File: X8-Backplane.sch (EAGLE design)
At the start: 16 parts, among them IC1 MAX3467CPA, U1 BD6221FSOP, U2 MIC29501-5.0WU, U3 MIC29501-5.0WU

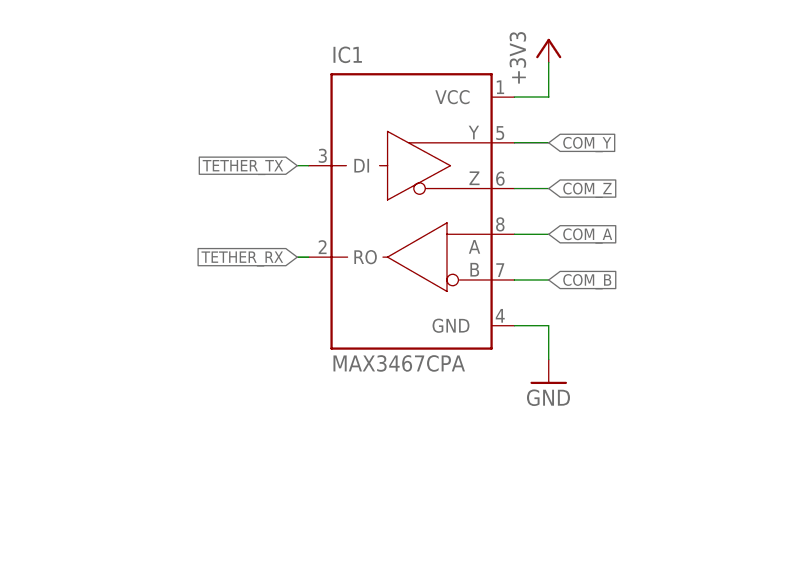
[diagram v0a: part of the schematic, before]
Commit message: finished adding components, added descriptions of pins
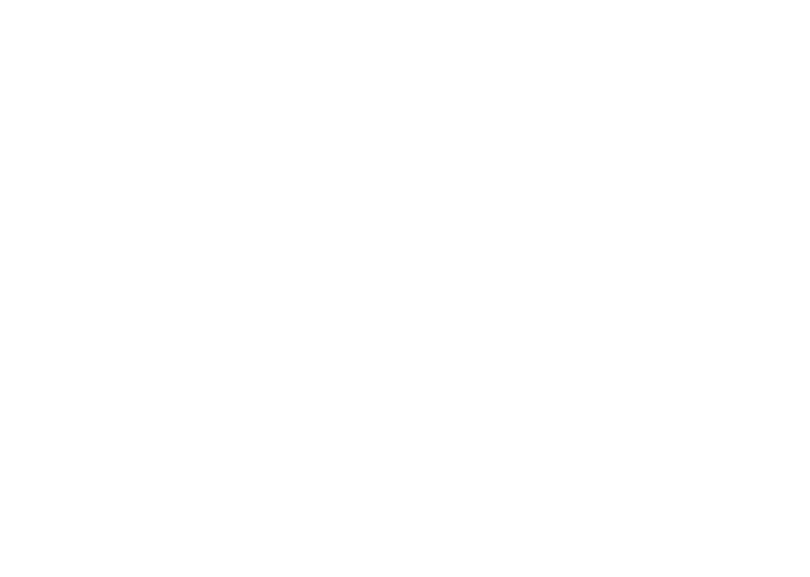
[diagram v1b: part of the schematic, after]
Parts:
- removed IC1: MAX3467CPA, maxim:MAX3467CPA
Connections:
- removed net +3V3: IC1.VCC
- removed net COM_A: IC1.A
- removed net COM_B: IC1.B
- removed net COM_Y: IC1.Y
- removed net COM_Z: IC1.Z
- removed net TETHER_RX: IC1.RO
- removed net TETHER_TX: IC1.DI
- net GND: no longer IC1.GND
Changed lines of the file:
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@@
 <part name="U$3" library="Other" deviceset="BNO055_9DOF_BREAKOUT" device=""/>
 <part name="U$4" library="backplane_to_shield_connector" deviceset="SHIELDCONNECTOR" device=""/>
-<part name="IC1" library="maxim" deviceset="MAX3467*" device="PA" technology="C"/>
-<part name="+3V1" library="supply1" deviceset="+3V3" device=""/>
-<part name="GND1" library="supply1" deviceset="GND" device=""/>
 <part name="U$7" library="test_lib" deviceset="PCA9615" device=""/>
 <part name="U2" library="LDO" deviceset="MIC29501-5.0WU" device=""/>
@@
 <instance part="U$4" gate="G$1" x="373.38" y="91.44"/>
 <instance part="U$4" gate="G$2" x="419.1" y="88.9"/>
-<instance part="IC1" gate="G$1" x="496.57" y="172.72"/>
-<instance part="+3V1" gate="G$1" x="513.08" y="191.77"/>
-<instance part="GND1" gate="1" x="513.08" y="153.67"/>
 <instance part="U$7" gate="G$1" x="408.94" y="165.1"/>
 <instance part="U2" gate="A" x="160.02" y="-40.64"/>
@@
 <nets>
 <net name="GND" class="0">
-<segment>
-<pinref part="IC1" gate="G$1" pin="GND"/>
-<wire x1="509.27" y1="160.02" x2="513.08" y2="160.02" width="0.1524" layer="91"/>
-<wire x1="513.08" y1="160.02" x2="513.08" y2="156.21" width="0.1524" layer="91"/>
-<pinref part="GND1" gate="1" pin="GND"/>
-</segment>
 <segment>
 <pinref part="U2" gate="A" pin="GND"/>
@@
 </segment>
 </net>
-<net name="+3V3" class="0">
-<segment>
-<pinref part="IC1" gate="G$1" pin="VCC"/>
-<wire x1="509.27" y1="185.42" x2="513.08" y2="185.42" width="0.1524" layer="91"/>
-<wire x1="513.08" y1="185.42" x2="513.08" y2="189.23" width="0.1524" layer="91"/>
-<pinref part="+3V1" gate="G$1" pin="+3V3"/>
-</segment>
-</net>
-<net name="TETHER_RX" class="0">
-<segment>
-<pinref part="IC1" gate="G$1" pin="RO"/>
-<wire x1="486.41" y1="167.64" x2="485.14" y2="167.64" width="0.1524" layer="91"/>
-<label x="485.14" y="167.64" size="1.27" layer="95" rot="R180" xref="yes"/>
-</segment>
-</net>
-<net name="TETHER_TX" class="0">
-<segment>
-<label x="485.14" y="177.8" size="1.27" layer="95" rot="R180" xref="yes"/>
-<pinref part="IC1" gate="G$1" pin="DI"/>
-<wire x1="485.14" y1="177.8" x2="486.41" y2="177.8" width="0.1524" layer="91"/>
-</segment>
-</net>
-<net name="COM_A" class="0">
-<segment>
-<pinref part="IC1" gate="G$1" pin="A"/>
-<wire x1="509.27" y1="170.18" x2="513.08" y2="170.18" width="0.1524" layer="91"/>
-<label x="513.08" y="170.18" size="1.27" layer="95" xref="yes"/>
-</segment>
-</net>
-<net name="COM_B" class="0">
-<segment>
-<pinref part="IC1" gate="G$1" pin="B"/>
-<wire x1="509.27" y1="165.1" x2="513.08" y2="165.1" width="0.1524" layer="91"/>
-<label x="513.08" y="165.1" size="1.27" layer="95" xref="yes"/>
-</segment>
-</net>
-<net name="COM_Y" class="0">
-<segment>
-<pinref part="IC1" gate="G$1" pin="Y"/>
-<wire x1="509.27" y1="180.34" x2="513.08" y2="180.34" width="0.1524" layer="91"/>
-<label x="513.08" y="180.34" size="1.27" layer="95" xref="yes"/>
-</segment>
-</net>
-<net name="COM_Z" class="0">
-<segment>
-<pinref part="IC1" gate="G$1" pin="Z"/>
-<wire x1="509.27" y1="175.26" x2="513.08" y2="175.26" width="0.1524" layer="91"/>
-<label x="513.08" y="175.26" size="1.27" layer="95" xref="yes"/>
-</segment>
-</net>
